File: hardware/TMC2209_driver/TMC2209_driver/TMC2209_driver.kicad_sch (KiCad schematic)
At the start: 21 parts, among them J1 Conn_01x08, J2 Conn_01x08, J3 Conn_01x02

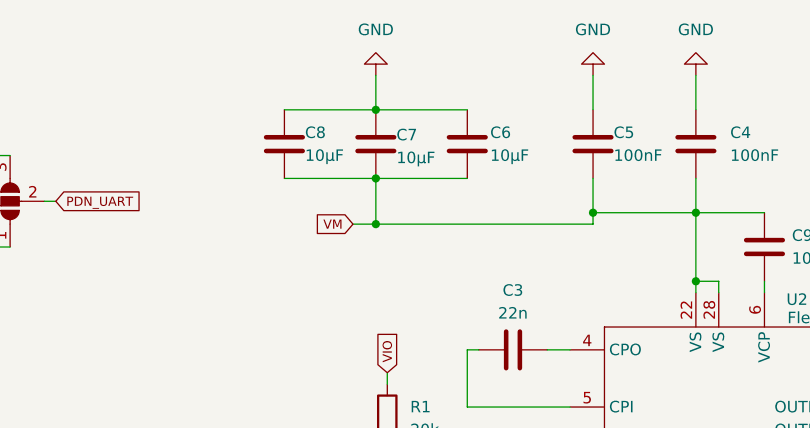
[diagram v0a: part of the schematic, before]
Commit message: finished driver board design
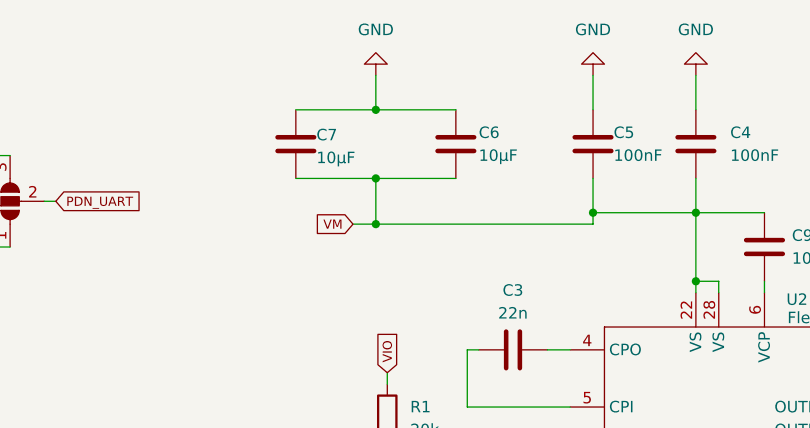
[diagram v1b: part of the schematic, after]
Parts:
- removed C8: 10µF, Capacitor_SMD:C_1206_3216Metric, symbol Device:C
- C1, C2, C3, C4, C5, C9: footprint Capacitor_SMD:C_0603_1608Metric -> Capacitor_SMD:C_0402_1005Metric
- JP1: footprint Jumper:SolderJumper-3_P1.3mm_Open_Pad1.0x1.5mm -> FlexPrint:SolderJumper_3Pads
- R1, R2, R6: footprint Resistor_SMD:R_0603_1608Metric -> Resistor_SMD:R_0402_1005Metric
- R4, R5: footprint Resistor_SMD:R_1206_3216Metric -> Resistor_SMD:R_0805_2012Metric
- RV1: footprint Potentiometer_SMD:Potentiometer_Bourns_3314J_Vertical -> FlexPrint:TRIMMER_3312J-1-203E
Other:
- moved on the sheet: C6, C7
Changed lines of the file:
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@@
 	(wire
 		(pts
-			(xy 63.5 97.79) (xy 66.04 97.79)
+			(xy 115.57 55.88) (xy 124.46 55.88)
 		)
 		(stroke
@@
 	(wire
 		(pts
-			(xy 179.07 119.38) (xy 186.69 119.38)
+			(xy 63.5 97.79) (xy 66.04 97.79)
 		)
 		(stroke
@@
 	(wire
 		(pts
-			(xy 63.5 66.04) (xy 66.04 66.04)
+			(xy 179.07 119.38) (xy 186.69 119.38)
 		)
 		(stroke
@@
 	(wire
 		(pts
-			(xy 114.3 55.88) (xy 124.46 55.88)
+			(xy 63.5 66.04) (xy 66.04 66.04)
 		)
 		(stroke
@@
 	(wire
 		(pts
-			(xy 114.3 48.26) (xy 124.46 48.26)
-		)
-		(stroke
-			(width 0)
-			(type default)
-		)
-	)
-	(wire
-		(pts
 			(xy 116.84 124.46) (xy 116.84 127)
 		)
@@
 	(wire
 		(pts
-			(xy 124.46 55.88) (xy 134.62 55.88)
+			(xy 124.46 55.88) (xy 133.35 55.88)
 		)
 		(stroke
@@
 	(wire
 		(pts
-			(xy 124.46 48.26) (xy 134.62 48.26)
+			(xy 124.46 48.26) (xy 133.35 48.26)
 		)
 		(stroke
@@
 	(wire
 		(pts
+			(xy 115.57 48.26) (xy 124.46 48.26)
+		)
+		(stroke
+			(width 0)
+			(type default)
+		)
+	)
+	(wire
+		(pts
 			(xy 142.24 99.06) (xy 146.05 99.06)
 		)
@@
 	(symbol
 		(lib_id "Device:C")
-		(at 124.46 52.07 0)
+		(at 115.57 52.07 0)
 		(unit 1)
 		(exclude_from_sim no)
@@
 		(dnp no)
 		(property "Reference" "C7"
-			(at 126.746 51.054 0)
+			(at 117.856 51.054 0)
 			(effects
 				(font
@@
 		)
 		(property "Value" "10µF"
-			(at 126.746 53.594 0)
+			(at 117.856 53.594 0)
 			(effects
 				(font
@@
 		)
 		(property "Footprint" "Capacitor_SMD:C_1206_3216Metric"
-			(at 125.4252 55.88 0)
+			(at 116.5352 55.88 0)
 			(effects
 				(font
@@
 		)
 		(property "Datasheet" "~"
-			(at 124.46 52.07 0)
+			(at 115.57 52.07 0)
 			(effects
 				(font
@@
 		)
 		(property "Description" "Unpolarized capacitor"
-			(at 124.46 52.07 0)
+			(at 115.57 52.07 0)
 			(effects
 				(font
@@
 			)
 		)
-		(property "Footprint" "Capacitor_SMD:C_0603_1608Metric"
+		(property "Footprint" "Capacitor_SMD:C_0402_1005Metric"
 			(at 187.6552 106.68 0)
 			(effects
@@
 			)
 		)
-		(property "Footprint" "Resistor_SMD:R_1206_3216Metric"
+		(property "Footprint" "Resistor_SMD:R_0805_2012Metric"
 			(at 192.532 123.19 90)
 			(effects
@@
 			)
 		)
-		(property "Footprint" "Resistor_SMD:R_0603_1608Metric"
+		(property "Footprint" "Resistor_SMD:R_0402_1005Metric"
 			(at 110.49 109.982 90)
 			(effects
@@
 			)
 		)
-		(property "Footprint" "Capacitor_SMD:C_0603_1608Metric"
+		(property "Footprint" "Capacitor_SMD:C_0402_1005Metric"
 			(at 143.51 73.9648 0)
 			(effects
@@
 			)
 		)
-		(property "Footprint" "Capacitor_SMD:C_0603_1608Metric"
+		(property "Footprint" "Capacitor_SMD:C_0402_1005Metric"
 			(at 160.9852 55.88 0)
 			(effects
@@
 			)
 		)
-		(property "Footprint" "Capacitor_SMD:C_0603_1608Metric"
+		(property "Footprint" "Capacitor_SMD:C_0402_1005Metric"
 			(at 195.2752 106.68 0)
 			(effects
@@
 			)
 		)
-		(property "Footprint" "Resistor_SMD:R_0603_1608Metric"
+		(property "Footprint" "Resistor_SMD:R_0402_1005Metric"
 			(at 127.762 120.65 90)
 			(effects
@@
 	)
 	(symbol
-		(lib_id "Device:C")
-		(at 114.3 52.07 0)
-		(unit 1)
-		(exclude_from_sim no)
-		(in_bom yes)
-		(on_board yes)
-		(dnp no)
-		(property "Reference" "C8"
-			(at 116.586 50.8 0)
-			(effects
-				(font
-					(size 1.27 1.27)
-				)
-				(justify left)
-			)
-		)
-		(property "Value" "10µF"
-			(at 116.586 53.34 0)
-			(effects
-				(font
-					(size 1.27 1.27)
-				)
-				(justify left)
-			)
-		)
-		(property "Footprint" "Capacitor_SMD:C_1206_3216Metric"
-			(at 115.2652 55.88 0)
-			(effects
-				(font
-					(size 1.27 1.27)
-				)
-				(hide yes)
-			)
-		)
-		(property "Datasheet" "~"
-			(at 114.3 52.07 0)
-			(effects
-				(font
-					(size 1.27 1.27)
-				)
-				(hide yes)
-			)
-		)
-		(property "Description" "Unpolarized capacitor"
-			(at 114.3 52.07 0)
-			(effects
-				(font
-					(size 1.27 1.27)
-				)
-				(hide yes)
-			)
-		)
-		(pin "1"
-		)
-		(pin "2"
-		)
-		(instances
-			(project ""
-				(path "/ffb67535-1c6e-42d2-9b3b-d74a0518d54b"
-					(reference "C8")
-					(unit 1)
-				)
-			)
-		)
-	)
-	(symbol
 		(lib_id "power:GND")
 		(at 186.69 129.54 0)
@@
 			)
 		)
-		(property "Footprint" "Capacitor_SMD:C_0603_1608Metric"
+		(property "Footprint" "Capacitor_SMD:C_0402_1005Metric"
 			(at 168.6052 67.31 0)
 			(effects
@@
 			)
 		)
-		(property "Footprint" "Resistor_SMD:R_0603_1608Metric"
+		(property "Footprint" "Resistor_SMD:R_0402_1005Metric"
 			(at 123.952 82.55 90)
 			(effects
@@
 			)
 		)
-		(property "Footprint" "Jumper:SolderJumper-3_P1.3mm_Open_Pad1.0x1.5mm"
+		(property "Footprint" "FlexPrint:SolderJumper_3Pads"
 			(at 83.82 58.42 0)
 			(effects
@@
 			)
 		)
-		(property "Footprint" "Potentiometer_SMD:Potentiometer_Bourns_3314J_Vertical"
+		(property "Footprint" "FlexPrint:TRIMMER_3312J-1-203E"
 			(at 116.84 120.65 0)
 			(effects
@@
 			)
 		)
-		(property "Footprint" "Resistor_SMD:R_1206_3216Metric"
+		(property "Footprint" "Resistor_SMD:R_0805_2012Metric"
 			(at 184.912 123.19 90)
 			(effects
@@
 			)
 		)
-		(property "Footprint" "Capacitor_SMD:C_0603_1608Metric"
+		(property "Footprint" "Capacitor_SMD:C_0402_1005Metric"
 			(at 149.5552 55.88 0)
 			(effects
@@
 	(symbol
 		(lib_id "Device:C")
-		(at 134.62 52.07 0)
+		(at 133.35 52.07 0)
 		(unit 1)
 		(exclude_from_sim no)
@@
 		(dnp no)
 		(property "Reference" "C6"
-			(at 137.16 50.8 0)
+			(at 135.89 50.8 0)
 			(effects
 				(font
@@
 		)
 		(property "Value" "10µF"
-			(at 137.16 53.34 0)
+			(at 135.89 53.34 0)
 			(effects
 				(font
@@
 		)
 		(property "Footprint" "Capacitor_SMD:C_1206_3216Metric"
-			(at 135.5852 55.88 0)
+			(at 134.3152 55.88 0)
 			(effects
 				(font
@@
 		)
 		(property "Datasheet" "~"
-			(at 134.62 52.07 0)
+			(at 133.35 52.07 0)
 			(effects
 				(font
@@
 		)
 		(property "Description" "Unpolarized capacitor"
-			(at 134.62 52.07 0)
+			(at 133.35 52.07 0)
 			(effects
 				(font
